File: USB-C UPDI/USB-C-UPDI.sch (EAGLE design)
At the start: 20 parts, among them IC1 FT232RL, J2 61300511121

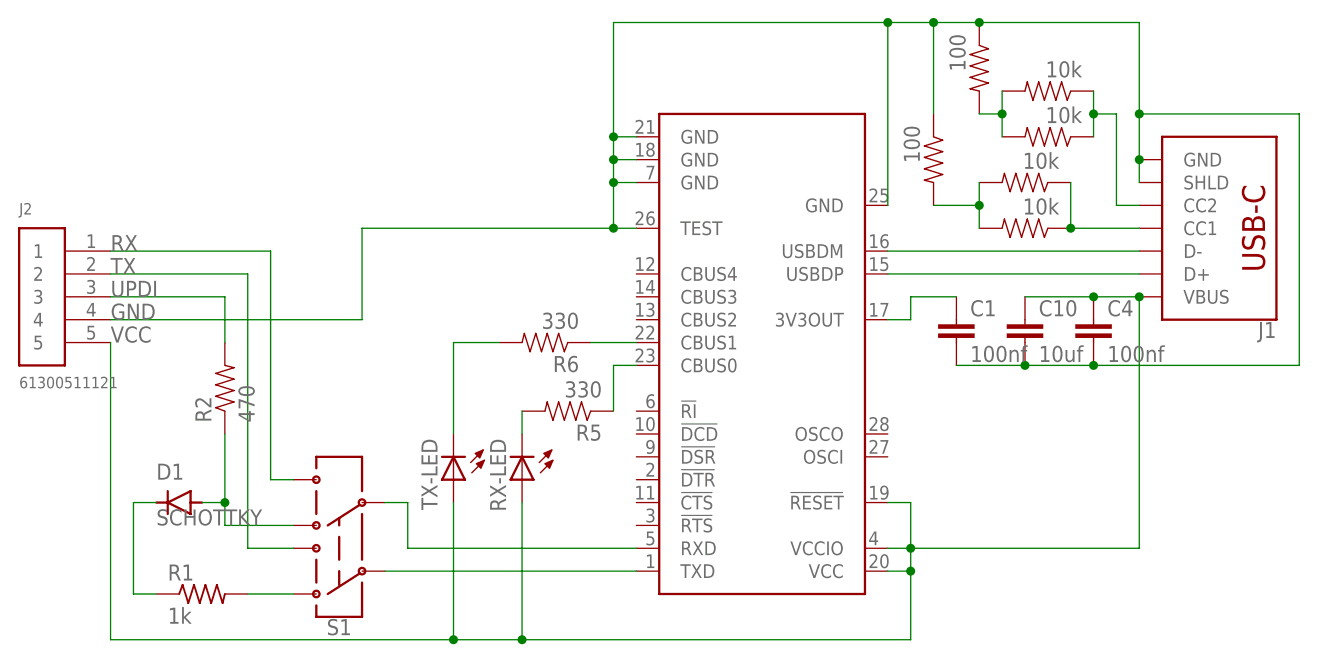
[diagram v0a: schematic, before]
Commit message: updates
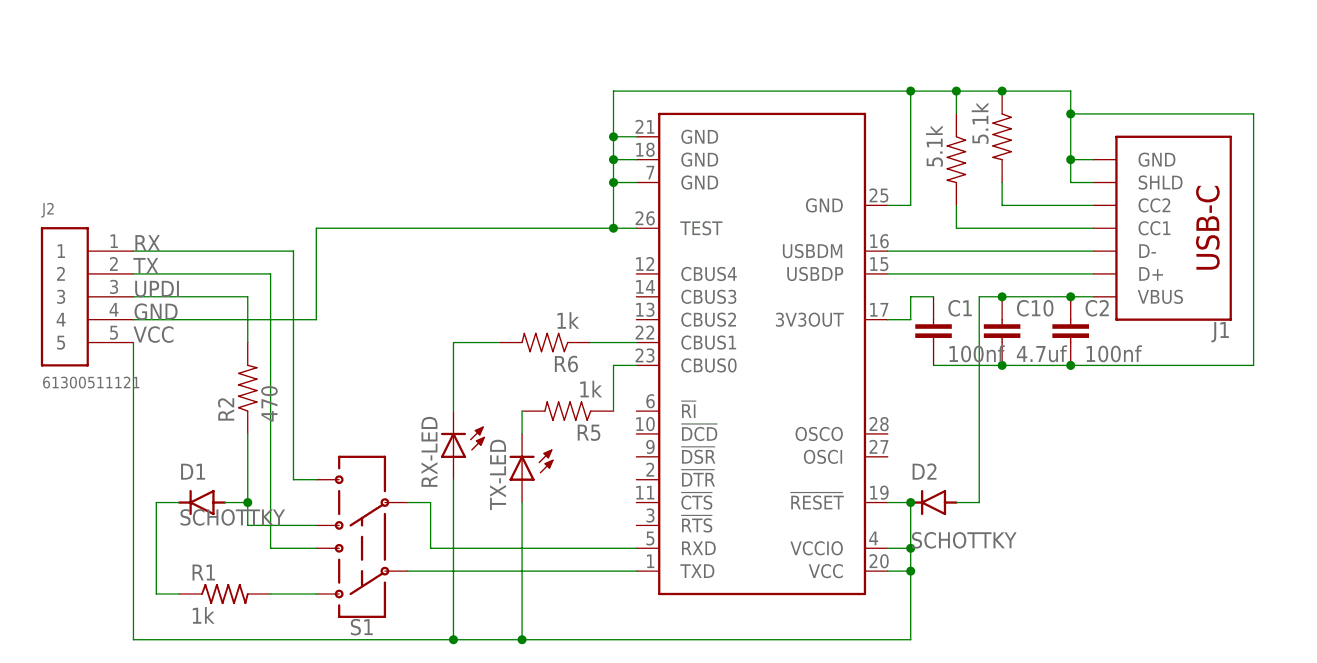
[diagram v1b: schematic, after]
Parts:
- removed C4: 100nf, 01_SparkFun:CAP1206
- removed R3, R4, R7, R8: 10k, 01_SparkFun:RESISTOR1206
- added C2: 100nf, 01_SparkFun:CAP1206
- added D2: SCHOTTKY, eagle_fab:DIODE_SCHOTTKY_CDBM1100-G
- C10: value 10uf -> 4.7uf
- R10, R9: value 100 -> 5.1k
- R5, R6: value 330 -> 1k
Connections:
- removed net N$50: R10.2, R3.2, R7.2
- net GND: now also C2.2; no longer C4.2
- net N$42: now also J1.CC2, R10.2; no longer R4.2, R8.2, R9.2
- net N$45: now also TX-LED.C; no longer RX-LED.C
- net N$46: now also RX-LED.C; no longer TX-LED.C
- net N$49: now also C10.1, C2.1, D2.ANODE, J1.VBUS; no longer J1.CC2, R3.1, R7.1
- net N$9: now also R9.2; no longer R4.1, R8.1
- net VCC: now also D2.KATHODE; no longer C10.1, C4.1, J1.VBUS
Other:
- moved on the sheet: C1, C10, D1, J1, J2, R1, R2, RX-LED, S1, TX-LED
